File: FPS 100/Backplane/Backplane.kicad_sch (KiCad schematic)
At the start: 11 parts, among them J2 Conn_02x50_100pin

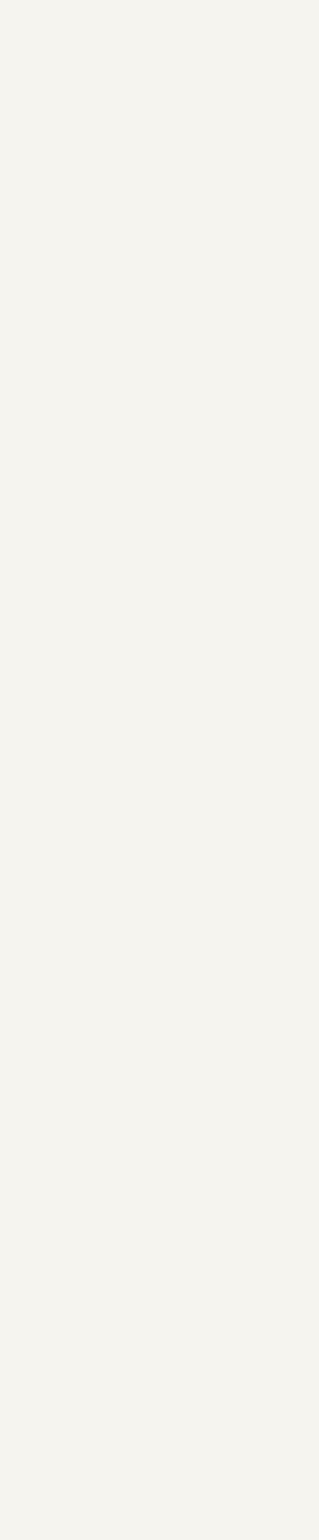
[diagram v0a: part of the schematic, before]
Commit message: 2026/1/2
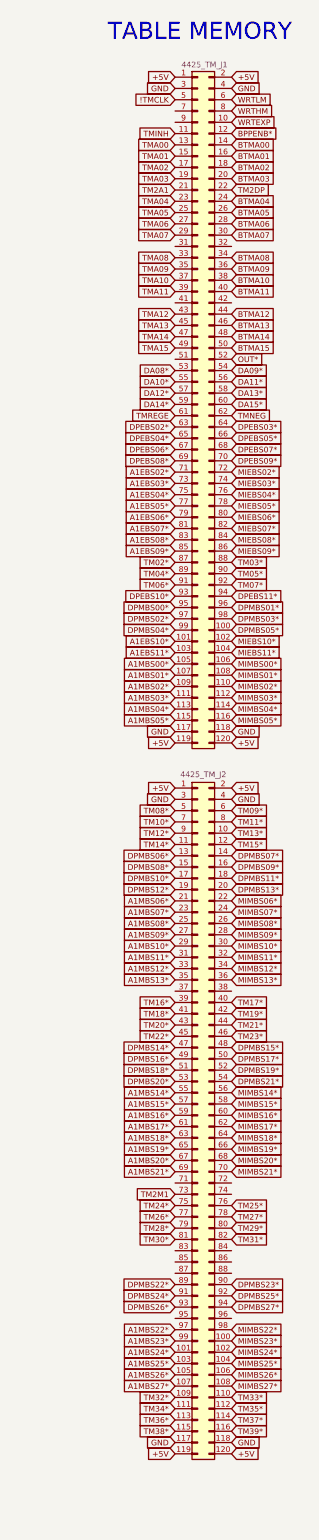
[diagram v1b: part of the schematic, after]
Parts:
- added 4425_TM_J1, 4425_TM_J2: Conn_02x60_120pin, symbol User:Conn_02x60_120pin
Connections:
- net +5V: now also 4425_TM_J1.1, 4425_TM_J1.119, 4425_TM_J1.120, 4425_TM_J1.2, 4425_TM_J2.1, 4425_TM_J2.119, 4425_TM_J2.120, 4425_TM_J2.2
- net A1EBS02*: now also 4425_TM_J1.71
- net A1EBS03*: now also 4425_TM_J1.73
- net A1EBS04*: now also 4425_TM_J1.75
- net A1EBS05*: now also 4425_TM_J1.77
- net A1EBS06*: now also 4425_TM_J1.79
- net A1EBS07*: now also 4425_TM_J1.81
- net A1EBS08*: now also 4425_TM_J1.83
- net A1EBS09*: now also 4425_TM_J1.85
- net A1EBS10*: now also 4425_TM_J1.101
- net A1EBS11*: now also 4425_TM_J1.103
- net A1MBS00*: now also 4425_TM_J1.105
- net A1MBS01*: now also 4425_TM_J1.107
- net A1MBS02*: now also 4425_TM_J1.109
- net A1MBS03*: now also 4425_TM_J1.111
- net A1MBS04*: now also 4425_TM_J1.113
- net A1MBS05*: now also 4425_TM_J1.115
- net A1MBS06*: now also 4425_TM_J2.21
- net A1MBS07*: now also 4425_TM_J2.23
- net A1MBS08*: now also 4425_TM_J2.25
- net A1MBS09*: now also 4425_TM_J2.27
- net A1MBS10*: now also 4425_TM_J2.29
- net A1MBS11*: now also 4425_TM_J2.31
- net A1MBS12*: now also 4425_TM_J2.33
- net A1MBS13*: now also 4425_TM_J2.35
- net A1MBS14*: now also 4425_TM_J2.55
- net A1MBS15*: now also 4425_TM_J2.57
- net A1MBS16*: now also 4425_TM_J2.59
- net A1MBS17*: now also 4425_TM_J2.61
- net A1MBS18*: now also 4425_TM_J2.63
- net A1MBS19*: now also 4425_TM_J2.65
- net A1MBS20*: now also 4425_TM_J2.67
- net A1MBS21*: now also 4425_TM_J2.69
- net A1MBS22*: now also 4425_TM_J2.97
- net A1MBS23*: now also 4425_TM_J2.99
- net A1MBS24*: now also 4425_TM_J2.101
- net A1MBS25*: now also 4425_TM_J2.103
- net A1MBS26*: now also 4425_TM_J2.105
- net A1MBS27*: now also 4425_TM_J2.107
- net DPEBS02*: now also 4425_TM_J1.63
- net DPEBS03*: now also 4425_TM_J1.64
- net DPEBS04*: now also 4425_TM_J1.65
- net DPEBS05*: now also 4425_TM_J1.66
- net DPEBS06*: now also 4425_TM_J1.67
- net DPEBS07*: now also 4425_TM_J1.68
- net DPEBS08*: now also 4425_TM_J1.69
- net DPEBS09*: now also 4425_TM_J1.70
- net DPEBS10*: now also 4425_TM_J1.93
- net DPEBS11*: now also 4425_TM_J1.94
- net DPMBS00*: now also 4425_TM_J1.95
- net DPMBS01*: now also 4425_TM_J1.96
- net DPMBS02*: now also 4425_TM_J1.97
- net DPMBS03*: now also 4425_TM_J1.98
- net DPMBS04*: now also 4425_TM_J1.99
- net DPMBS05*: now also 4425_TM_J1.100
- net DPMBS06*: now also 4425_TM_J2.13
- net DPMBS07*: now also 4425_TM_J2.14
- net DPMBS08*: now also 4425_TM_J2.15
- net DPMBS09*: now also 4425_TM_J2.16
- net DPMBS10*: now also 4425_TM_J2.17
- net DPMBS11*: now also 4425_TM_J2.18
- net DPMBS12*: now also 4425_TM_J2.19
- net DPMBS13*: now also 4425_TM_J2.20
- net DPMBS14*: now also 4425_TM_J2.47
- net DPMBS15*: now also 4425_TM_J2.48
- net DPMBS17*: now also 4425_TM_J2.50
- net DPMBS18*: now also 4425_TM_J2.51
- net DPMBS19*: now also 4425_TM_J2.52
- net DPMBS20*: now also 4425_TM_J2.53
- net DPMBS21*: now also 4425_TM_J2.54
- net DPMBS22*: now also 4425_TM_J2.89
- net DPMBS24*: now also 4425_TM_J2.91
- net DPMBS25*: now also 4425_TM_J2.92
- net DPMBS26*: now also 4425_TM_J2.93
- net DPMBS27*: now also 4425_TM_J2.94
- net GND: now also 4425_TM_J1.117, 4425_TM_J1.118, 4425_TM_J1.3, 4425_TM_J1.4, 4425_TM_J2.117, 4425_TM_J2.118, 4425_TM_J2.3, 4425_TM_J2.4
- net WRTEXP: now also 4425_TM_J1.10
- net WRTHM: now also 4425_TM_J1.8
- net WRTLM: now also 4425_TM_J1.6
- new net !TMCLK: 4425_TM_J1.5
- new net BPPENB*: 4425_TM_J1.12
- new net BTMA00: 4425_TM_J1.14
- new net BTMA01: 4425_TM_J1.16
- new net BTMA02: 4425_TM_J1.18
- new net BTMA03: 4425_TM_J1.20
- new net BTMA04: 4425_TM_J1.24
- new net BTMA05: 4425_TM_J1.26
- new net BTMA06: 4425_TM_J1.28
- new net BTMA07: 4425_TM_J1.30
- new net BTMA08: 4425_TM_J1.34
- new net BTMA09: 4425_TM_J1.36
- new net BTMA10: 4425_TM_J1.38
- new net BTMA11: 4425_TM_J1.40
- new net BTMA12: 4425_TM_J1.44
- new net BTMA13: 4425_TM_J1.46
- new net BTMA14: 4425_TM_J1.48
- new net BTMA15: 4425_TM_J1.50
- new net DA08*: 4425_TM_J1.53
- new net DA09*: 4425_TM_J1.54
- new net DA10*: 4425_TM_J1.55
- new net DA11*: 4425_TM_J1.56
- new net DA12*: 4425_TM_J1.57
- new net DA13*: 4425_TM_J1.58
- new net DA14*: 4425_TM_J1.59
- new net DA15*: 4425_TM_J1.60
- new net DPMBS16*: 4425_TM_J2.49
- new net DPMBS23*: 4425_TM_J2.90
- new net MIEBS02*: 4425_TM_J1.72
- new net MIEBS03*: 4425_TM_J1.74
- new net MIEBS04*: 4425_TM_J1.76
- new net MIEBS05*: 4425_TM_J1.78
- new net MIEBS06*: 4425_TM_J1.80
- new net MIEBS07*: 4425_TM_J1.82
- new net MIEBS08*: 4425_TM_J1.84
- new net MIEBS09*: 4425_TM_J1.86
- new net MIEBS10*: 4425_TM_J1.102
- new net MIEBS11*: 4425_TM_J1.104
- new net MIMBS00*: 4425_TM_J1.106
- new net MIMBS01*: 4425_TM_J1.108
- new net MIMBS02*: 4425_TM_J1.110
- new net MIMBS03*: 4425_TM_J1.112
- new net MIMBS04*: 4425_TM_J1.114
- new net MIMBS05*: 4425_TM_J1.116
- new net MIMBS06*: 4425_TM_J2.22
- new net MIMBS07*: 4425_TM_J2.24
- new net MIMBS08*: 4425_TM_J2.26
- new net MIMBS09*: 4425_TM_J2.28
- new net MIMBS10*: 4425_TM_J2.30
- new net MIMBS11*: 4425_TM_J2.32
- new net MIMBS12*: 4425_TM_J2.34
- new net MIMBS13*: 4425_TM_J2.36
- new net MIMBS14*: 4425_TM_J2.56
- new net MIMBS15*: 4425_TM_J2.58
- new net MIMBS16*: 4425_TM_J2.60
- new net MIMBS17*: 4425_TM_J2.62
- new net MIMBS18*: 4425_TM_J2.64
- new net MIMBS19*: 4425_TM_J2.66
- new net MIMBS20*: 4425_TM_J2.68
- new net MIMBS21*: 4425_TM_J2.70
- new net MIMBS22*: 4425_TM_J2.98
- new net MIMBS23*: 4425_TM_J2.100
- new net MIMBS24*: 4425_TM_J2.102
- new net MIMBS25*: 4425_TM_J2.104
- new net MIMBS26*: 4425_TM_J2.106
- new net MIMBS27*: 4425_TM_J2.108
- new net OUT*: 4425_TM_J1.52
- new net TM02*: 4425_TM_J1.87
- new net TM03*: 4425_TM_J1.88
- new net TM04*: 4425_TM_J1.89
- new net TM05*: 4425_TM_J1.90
- new net TM06*: 4425_TM_J1.91
- new net TM07*: 4425_TM_J1.92
- new net TM08*: 4425_TM_J2.5
- new net TM09*: 4425_TM_J2.6
- new net TM10*: 4425_TM_J2.7
- new net TM11*: 4425_TM_J2.8
- new net TM12*: 4425_TM_J2.9
- new net TM13*: 4425_TM_J2.10
- new net TM14*: 4425_TM_J2.11
- new net TM15*: 4425_TM_J2.12
- new net TM16*: 4425_TM_J2.39
- new net TM17*: 4425_TM_J2.40
- new net TM18*: 4425_TM_J2.41
- new net TM19*: 4425_TM_J2.42
- new net TM20*: 4425_TM_J2.43
- new net TM21*: 4425_TM_J2.44
- new net TM22*: 4425_TM_J2.45
- new net TM23*: 4425_TM_J2.46
- new net TM24*: 4425_TM_J2.75
- new net TM25*: 4425_TM_J2.76
- new net TM26*: 4425_TM_J2.77
- new net TM27*: 4425_TM_J2.78
- new net TM28*: 4425_TM_J2.79
- new net TM29*: 4425_TM_J2.80
- new net TM2A1: 4425_TM_J1.21
- new net TM2DP: 4425_TM_J1.22
- new net TM2M1: 4425_TM_J2.73
- new net TM30*: 4425_TM_J2.81
- new net TM31*: 4425_TM_J2.82
- new net TM32*: 4425_TM_J2.109
- new net TM33*: 4425_TM_J2.110
- new net TM34*: 4425_TM_J2.111
- new net TM35*: 4425_TM_J2.112
- new net TM36*: 4425_TM_J2.113
- new net TM37*: 4425_TM_J2.114
- new net TM38*: 4425_TM_J2.115
- new net TM39*: 4425_TM_J2.116
- new net TMA00: 4425_TM_J1.13
- new net TMA01: 4425_TM_J1.15
- new net TMA02: 4425_TM_J1.17
- new net TMA03: 4425_TM_J1.19
- new net TMA04: 4425_TM_J1.23
- new net TMA05: 4425_TM_J1.25
- new net TMA06: 4425_TM_J1.27
- new net TMA07: 4425_TM_J1.29
- new net TMA08: 4425_TM_J1.33
- new net TMA09: 4425_TM_J1.35
- new net TMA10: 4425_TM_J1.37
- new net TMA11: 4425_TM_J1.39
- new net TMA12: 4425_TM_J1.43
- new net TMA13: 4425_TM_J1.45
- new net TMA14: 4425_TM_J1.47
- new net TMA15: 4425_TM_J1.49
- new net TMINH: 4425_TM_J1.11
- new net TMNEG: 4425_TM_J1.62
- new net TMREGE: 4425_TM_J1.61
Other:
- note added: "TABLE MEMORY"
